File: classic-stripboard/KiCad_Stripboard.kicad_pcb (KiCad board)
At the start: 2 copper layers, 95 x 130 mm, 372 parts

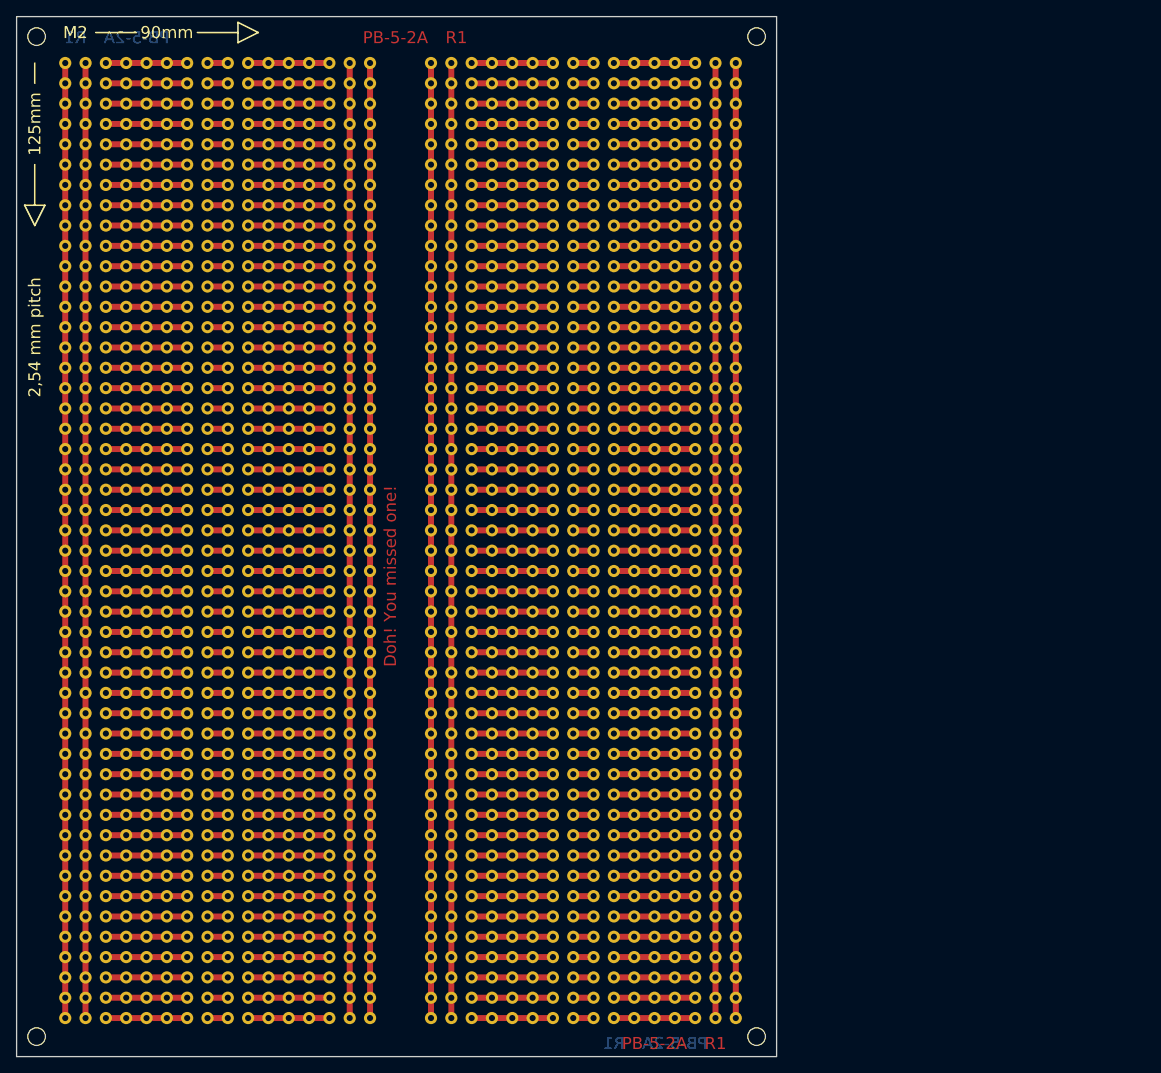
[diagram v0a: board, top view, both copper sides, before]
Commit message: initial commit
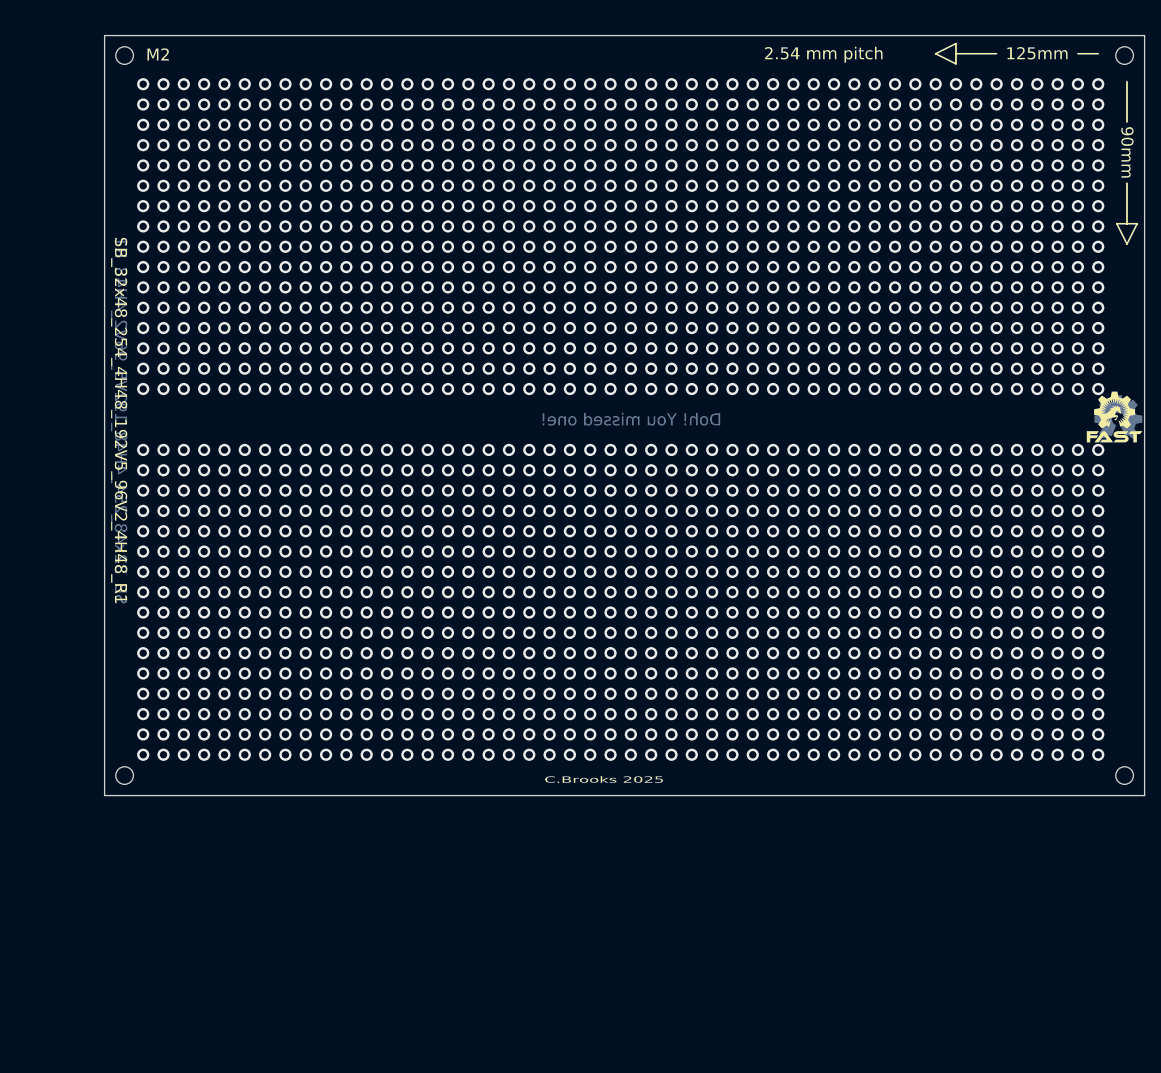
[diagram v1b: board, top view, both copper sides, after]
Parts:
- removed the REF** at (137.2, 50.8)
- removed the REF** at (137.2, 73.7)
- removed the REF** at (119.4, 167.6)
- removed the REF** at (119.4, 162.6)
- removed the REF** at (119.4, 149.9)
- removed the REF** at (119.4, 152.4)
- removed the REF** at (119.4, 147.3)
- removed the REF** at (119.4, 142.2)
- removed the REF** at (119.4, 144.8)
- removed the REF** at (119.4, 157.5)
- removed the REF** at (119.4, 154.9)
- removed the REF** at (119.4, 139.7)
- removed the REF** at (137.2, 76.2)
- removed the REF** at (119.4, 63.5)
- removed the REF** at (119.4, 68.6)
- removed the REF** at (119.4, 66.0)
- removed the REF** at (119.4, 71.1)
- removed the REF** at (119.4, 73.7)
- removed the REF** at (119.4, 58.4)
- removed the REF** at (119.4, 55.9)
- removed the REF** at (119.4, 53.3)
- removed the REF** at (119.4, 50.8)
- removed the REF** at (119.4, 61.0)
- removed the REF** at (137.2, 78.7)
- removed the REF** at (119.4, 96.5)
- removed the REF** at (119.4, 94.0)
- removed the REF** at (119.4, 99.1)
- removed the REF** at (119.4, 91.4)
- removed the REF** at (119.4, 101.6)
- removed the REF** at (119.4, 88.9)
- removed the REF** at (119.4, 86.4)
- removed the REF** at (119.4, 83.8)
- removed the REF** at (119.4, 81.3)
- removed the REF** at (119.4, 78.7)
- removed the REF** at (137.2, 106.7)
- removed the REF** at (119.4, 76.2)
- removed the REF** at (119.4, 109.2)
- removed the REF** at (119.4, 111.8)
- removed the REF** at (119.4, 116.8)
- removed the REF** at (119.4, 114.3)
- removed the REF** at (119.4, 119.4)
- removed the REF** at (119.4, 129.5)
- removed the REF** at (119.4, 124.5)
- removed the REF** at (119.4, 132.1)
- removed the REF** at (119.4, 121.9)
- removed the REF** at (137.2, 109.2)
- removed the REF** at (119.4, 127.0)
- removed the REF** at (119.4, 106.7)
- removed the REF** at (119.4, 104.1)
- removed the REF** at (119.4, 134.6)
- removed the REF** at (119.4, 137.2)
- removed the REF** at (149.9, 61.0)
- removed the REF** at (149.9, 73.7)
- removed the REF** at (149.9, 86.4)
- removed the REF** at (149.9, 99.1)
- removed the REF** at (149.9, 111.8)
- removed the REF** at (137.2, 91.4)
- removed the REF** at (149.9, 124.5)
- removed the REF** at (149.9, 137.2)
- removed the REF** at (149.9, 149.9)
- removed the REF** at (149.9, 162.6)
- removed the REF** at (149.9, 170.2)
- removed the REF** at (152.4, 162.6)
- removed the REF** at (152.4, 170.2)
- removed the REF** at (152.4, 149.9)
- removed the REF** at (152.4, 73.7)
- removed the REF** at (152.4, 61.0)
- removed the REF** at (137.2, 94.0)
- removed the REF** at (152.4, 86.4)
- removed the REF** at (152.4, 99.1)
- removed the REF** at (152.4, 137.2)
- removed the REF** at (152.4, 124.5)
- removed the REF** at (152.4, 111.8)
- removed the REF** at (114.3, 162.6)
- removed the REF** at (116.8, 162.6)
- removed the REF** at (114.3, 170.2)
- removed the REF** at (116.8, 170.2)
- removed the REF** at (114.3, 149.9)
- removed the REF** at (137.2, 99.1)
- removed the REF** at (116.8, 149.9)
- removed the REF** at (114.3, 73.7)
- removed the REF** at (116.8, 73.7)
- removed the REF** at (114.3, 61.0)
- removed the REF** at (116.8, 61.0)
- removed the REF** at (114.3, 86.4)
- removed the REF** at (116.8, 86.4)
- removed the REF** at (114.3, 99.1)
- removed the REF** at (116.8, 99.1)
- removed the REF** at (114.3, 137.2)
- removed the REF** at (137.2, 104.1)
- removed the REF** at (116.8, 137.2)
- removed the REF** at (114.3, 124.5)
- removed the REF** at (116.8, 124.5)
- removed the REF** at (114.3, 111.8)
- removed the REF** at (116.8, 111.8)
- removed the REF** at (91.4, 86.4)
- removed the REF** at (104.1, 86.4)
- removed the REF** at (91.4, 78.7)
- removed the REF** at (91.4, 81.3)
- removed the REF** at (106.7, 86.4)
- removed the REF** at (137.2, 101.6)
- removed the REF** at (91.4, 76.2)
- removed the REF** at (91.4, 83.8)
- removed the REF** at (91.4, 58.4)
- removed the REF** at (86.4, 50.8)
- removed the REF** at (86.4, 53.3)
- removed the REF** at (86.4, 58.4)
- removed the REF** at (86.4, 55.9)
- removed the REF** at (86.4, 61.0)
- removed the REF** at (91.4, 50.8)
- removed the REF** at (104.1, 61.0)
- removed the REF** at (137.2, 53.3)
- removed the REF** at (137.2, 96.5)
- removed the REF** at (106.7, 61.0)
- removed the REF** at (91.4, 53.3)
- removed the REF** at (91.4, 55.9)
- removed the REF** at (91.4, 68.6)
- removed the REF** at (91.4, 61.0)
- removed the REF** at (106.7, 73.7)
- removed the REF** at (91.4, 63.5)
- removed the REF** at (91.4, 71.1)
- removed the REF** at (91.4, 66.0)
- removed the REF** at (104.1, 73.7)
- removed the REF** at (137.2, 81.3)
- removed the REF** at (91.4, 73.7)
- removed the REF** at (86.4, 66.0)
- removed the REF** at (86.4, 68.6)
- removed the REF** at (86.4, 73.7)
- removed the REF** at (86.4, 63.5)
- removed the REF** at (91.4, 142.2)
- removed the REF** at (91.4, 147.3)
- removed the REF** at (91.4, 139.7)
- removed the REF** at (104.1, 149.9)
- removed the REF** at (106.7, 149.9)
- removed the REF** at (137.2, 86.4)
- removed the REF** at (91.4, 144.8)
- removed the REF** at (73.7, 142.2)
- removed the REF** at (68.6, 149.9)
- removed the REF** at (73.7, 139.7)
- removed the REF** at (73.7, 144.8)
- removed the REF** at (71.1, 149.9)
- removed the REF** at (73.7, 147.3)
- removed the REF** at (86.4, 132.1)
- removed the REF** at (86.4, 129.5)
- removed the REF** at (86.4, 134.6)
- removed the REF** at (137.2, 88.9)
- removed the REF** at (86.4, 137.2)
- removed the REF** at (86.4, 139.7)
- removed the REF** at (86.4, 142.2)
- removed the REF** at (86.4, 144.8)
- removed the REF** at (86.4, 147.3)
- removed the REF** at (91.4, 132.1)
- removed the REF** at (91.4, 129.5)
- removed the REF** at (91.4, 134.6)
- removed the REF** at (91.4, 137.2)
- removed the REF** at (104.1, 137.2)
- removed the REF** at (137.2, 83.8)
- removed the REF** at (106.7, 137.2)
- removed the REF** at (91.4, 127.0)
- removed the REF** at (73.7, 127.0)
- removed the REF** at (73.7, 129.5)
- removed the REF** at (73.7, 132.1)
- removed the REF** at (86.4, 127.0)
- removed the REF** at (73.7, 134.6)
- removed the REF** at (71.1, 137.2)
- removed the REF** at (68.6, 137.2)
- removed the REF** at (73.7, 137.2)
- removed the REF** at (137.2, 154.9)
- removed the REF** at (91.4, 157.5)
- removed the REF** at (91.4, 160.0)
- removed the REF** at (91.4, 149.9)
- removed the REF** at (91.4, 152.4)
- removed the REF** at (91.4, 154.9)
- removed the REF** at (86.4, 167.6)
- removed the REF** at (91.4, 165.1)
- removed the REF** at (91.4, 170.2)
- removed the REF** at (86.4, 170.2)
- removed the REF** at (91.4, 167.6)
- removed the REF** at (137.2, 147.3)
- removed the REF** at (86.4, 165.1)
- removed the REF** at (73.7, 170.2)
- removed the REF** at (86.4, 162.6)
- removed the REF** at (86.4, 160.0)
- removed the REF** at (73.7, 167.6)
- removed the REF** at (68.6, 170.2)
- removed the REF** at (71.1, 170.2)
- removed the REF** at (73.7, 165.1)
- removed the REF** at (73.7, 157.5)
- removed the REF** at (68.6, 162.6)
- removed the REF** at (137.2, 149.9)
- removed the REF** at (73.7, 154.9)
- removed the REF** at (73.7, 149.9)
- removed the REF** at (73.7, 152.4)
- removed the REF** at (71.1, 162.6)
- removed the REF** at (73.7, 162.6)
- removed the REF** at (73.7, 160.0)
- removed the REF** at (104.1, 170.2)
- removed the REF** at (104.1, 162.6)
- removed the REF** at (106.7, 170.2)
- removed the REF** at (91.4, 162.6)
- removed the REF** at (137.2, 152.4)
- removed the REF** at (106.7, 162.6)
- removed the REF** at (86.4, 152.4)
- removed the REF** at (86.4, 154.9)
- removed the REF** at (86.4, 157.5)
- removed the REF** at (86.4, 149.9)
- removed the REF** at (91.4, 106.7)
- removed the REF** at (104.1, 111.8)
- removed the REF** at (106.7, 111.8)
- removed the REF** at (91.4, 109.2)
- removed the REF** at (91.4, 111.8)
- removed the REF** at (137.2, 157.5)
- removed the REF** at (91.4, 104.1)
- removed the REF** at (91.4, 101.6)
- removed the REF** at (86.4, 111.8)
- removed the REF** at (86.4, 109.2)
- removed the REF** at (86.4, 114.3)
- removed the REF** at (86.4, 101.6)
- removed the REF** at (86.4, 96.5)
- removed the REF** at (86.4, 106.7)
- removed the REF** at (86.4, 104.1)
- removed the REF** at (86.4, 99.1)
- removed the REF** at (137.2, 55.9)
- removed the REF** at (137.2, 114.3)
- removed the REF** at (86.4, 124.5)
- removed the REF** at (91.4, 114.3)
- removed the REF** at (104.1, 124.5)
- removed the REF** at (106.7, 124.5)
- removed the REF** at (91.4, 119.4)
- removed the REF** at (91.4, 116.8)
- removed the REF** at (91.4, 121.9)
- removed the REF** at (91.4, 124.5)
- removed the REF** at (91.4, 99.1)
- removed the REF** at (104.1, 99.1)
- removed the REF** at (137.2, 116.8)
- removed the REF** at (106.7, 99.1)
- removed the REF** at (91.4, 96.5)
- removed the REF** at (91.4, 91.4)
- removed the REF** at (91.4, 94.0)
- removed the REF** at (86.4, 91.4)
- removed the REF** at (86.4, 88.9)
- removed the REF** at (86.4, 94.0)
- removed the REF** at (91.4, 88.9)
- removed the REF** at (73.7, 119.4)
- removed the REF** at (73.7, 116.8)
- removed the REF** at (137.2, 111.8)
- removed the REF** at (73.7, 121.9)
- removed the REF** at (73.7, 114.3)
- removed the REF** at (73.7, 124.5)
- removed the REF** at (86.4, 116.8)
- removed the REF** at (86.4, 119.4)
- removed the REF** at (86.4, 121.9)
- removed the REF** at (73.7, 88.9)
- removed the REF** at (73.7, 94.0)
- removed the REF** at (73.7, 91.4)
- removed the REF** at (73.7, 99.1)
- removed the REF** at (137.2, 119.4)
- removed the REF** at (68.6, 99.1)
- removed the REF** at (71.1, 99.1)
- removed the REF** at (73.7, 96.5)
- removed the REF** at (73.7, 106.7)
- removed the REF** at (73.7, 111.8)
- removed the REF** at (73.7, 109.2)
- removed the REF** at (73.7, 104.1)
- removed the REF** at (73.7, 101.6)
- removed the REF** at (71.1, 111.8)
- removed the REF** at (68.6, 111.8)
- removed the REF** at (137.2, 127.0)
- removed the REF** at (71.1, 124.5)
- removed the REF** at (68.6, 124.5)
- removed the REF** at (86.4, 76.2)
- removed the REF** at (86.4, 78.7)
- removed the REF** at (86.4, 83.8)
- removed the REF** at (86.4, 71.1)
- removed the REF** at (86.4, 81.3)
- removed the REF** at (86.4, 86.4)
- removed the REF** at (71.1, 73.7)
- removed the REF** at (73.7, 71.1)
- removed the REF** at (137.2, 132.1)
- removed the REF** at (73.7, 66.0)
- removed the REF** at (68.6, 73.7)
- removed the REF** at (73.7, 73.7)
- removed the REF** at (73.7, 68.6)
- removed the REF** at (73.7, 63.5)
- removed the REF** at (73.7, 50.8)
- removed the REF** at (73.7, 61.0)
- removed the REF** at (71.1, 61.0)
- removed the REF** at (68.6, 61.0)
- removed the REF** at (73.7, 53.3)
- removed the REF** at (137.2, 129.5)
- removed the REF** at (73.7, 55.9)
- removed the REF** at (73.7, 58.4)
- removed the REF** at (71.1, 86.4)
- removed the REF** at (68.6, 86.4)
- removed the REF** at (73.7, 83.8)
- removed the REF** at (73.7, 86.4)
- removed the REF** at (73.7, 81.3)
- removed the REF** at (73.7, 76.2)
- removed the REF** at (73.7, 78.7)
- removed the REF** at (137.2, 124.5)
- removed the REF** at (137.2, 121.9)
- removed the REF** at (137.2, 142.2)
- removed the REF** at (137.2, 58.4)
- removed the REF** at (137.2, 137.2)
- removed the REF** at (137.2, 139.7)
- removed the REF** at (137.2, 134.6)
- removed the REF** at (137.2, 144.8)
- removed the REF** at (137.2, 162.6)
- removed the REF** at (137.2, 167.6)
- removed the REF** at (137.2, 170.2)
- removed the REF** at (137.2, 165.1)
- removed the REF** at (137.2, 160.0)
- removed the REF** at (132.1, 50.8)
- removed the REF** at (137.2, 61.0)
- removed the REF** at (132.1, 53.3)
- removed the REF** at (132.1, 55.9)
- removed the REF** at (132.1, 58.4)
- removed the REF** at (132.1, 61.0)
- removed the REF** at (132.1, 63.5)
- removed the REF** at (132.1, 78.7)
- removed the REF** at (132.1, 76.2)
- removed the REF** at (132.1, 71.1)
- removed the REF** at (132.1, 66.0)
- removed the REF** at (132.1, 68.6)
- removed the REF** at (137.2, 63.5)
- removed the REF** at (132.1, 73.7)
- removed the REF** at (132.1, 104.1)
- removed the REF** at (132.1, 106.7)
- removed the REF** at (132.1, 109.2)
- removed the REF** at (132.1, 91.4)
- removed the REF** at (132.1, 101.6)
- removed the REF** at (132.1, 94.0)
- removed the REF** at (132.1, 96.5)
- removed the REF** at (132.1, 99.1)
- removed the REF** at (132.1, 88.9)
- removed the REF** at (137.2, 66.0)
- removed the REF** at (132.1, 83.8)
- removed the REF** at (132.1, 86.4)
- removed the REF** at (132.1, 81.3)
- removed the REF** at (132.1, 170.2)
- removed the REF** at (132.1, 167.6)
- removed the REF** at (132.1, 165.1)
- removed the REF** at (132.1, 129.5)
- removed the REF** at (132.1, 127.0)
- removed the REF** at (132.1, 124.5)
- removed the REF** at (132.1, 121.9)
- removed the REF** at (137.2, 68.6)
- removed the REF** at (132.1, 111.8)
- removed the REF** at (132.1, 114.3)
- removed the REF** at (132.1, 119.4)
- removed the REF** at (132.1, 116.8)
- removed the REF** at (132.1, 139.7)
- removed the REF** at (132.1, 137.2)
- removed the REF** at (132.1, 132.1)
- removed the REF** at (132.1, 134.6)
- removed the REF** at (132.1, 144.8)
- removed the REF** at (132.1, 149.9)
- removed the REF** at (137.2, 71.1)
- removed the REF** at (132.1, 147.3)
- removed the REF** at (132.1, 142.2)
- removed the REF** at (132.1, 152.4)
- removed the REF** at (132.1, 154.9)
- removed the REF** at (132.1, 162.6)
- removed the REF** at (132.1, 157.5)
- removed the REF** at (132.1, 160.0)
- removed the REF** at (119.4, 165.1)
- removed the REF** at (119.4, 170.2)
- removed the REF** at (119.4, 160.0)
- added G***: LOGO, kml-custom:FAST-Logo-Small, F.Cu at (199.8, 94.9)
- added Ref**: Val**, kml-custom:OSHW_Logo_6mm, F.Cu at (200.2, 95.3)
- moved REF** 136.0 mm to (201.0, 49.9), turned to -90 degrees
- moved REF** 123.1 mm to (76.0, 49.9), turned to -90 degrees
- moved REF** 103.2 mm to (201.0, 139.9), turned to -90 degrees
- moved REF** 85.5 mm to (76.0, 139.9), turned to -90 degrees
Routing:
- net (no net): vias 0 -> 1536
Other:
- board size 95 x 130 mm -> 130 x 95 mm
- board text added: "2.54 mm pitch"
- board text added: "C.Brooks 2025"
- board text added: "SB_32x48_254_4H48_192V5_96V2_4H48_R1"
- board text removed: "2,54 mm pitch"
- board text removed: "PB-5-2A"
- board text removed: "R1"
